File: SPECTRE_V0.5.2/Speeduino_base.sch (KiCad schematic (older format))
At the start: 218 parts, among them J1 Conn_01x06_Male, J2 Conn_02x04_Odd_Even, J3 ProtoArea, Q1 AO3400, Q10 BSP78, Q11 BSP78, Q12 AO3400, Q13 BSP78, Q14 BSP78, Q15 BSP78, Q16 BSP78, Q17 BSP78, Q18 BSP78, Q19 BSP78, Q20 BSP78, Q21 BSP78, Q6 AO3400, Q7 AO3400, Q8 AO3400, Q9 AO3400, U1 MAX9926UAEE+, U2 LM78M05_TO220, U3 TL431DBZ, U4 molex_48pin, U5 TJA1050, U6 MAX3232, U7 MIC4427, U8 MIC4427, U9 MIC4427

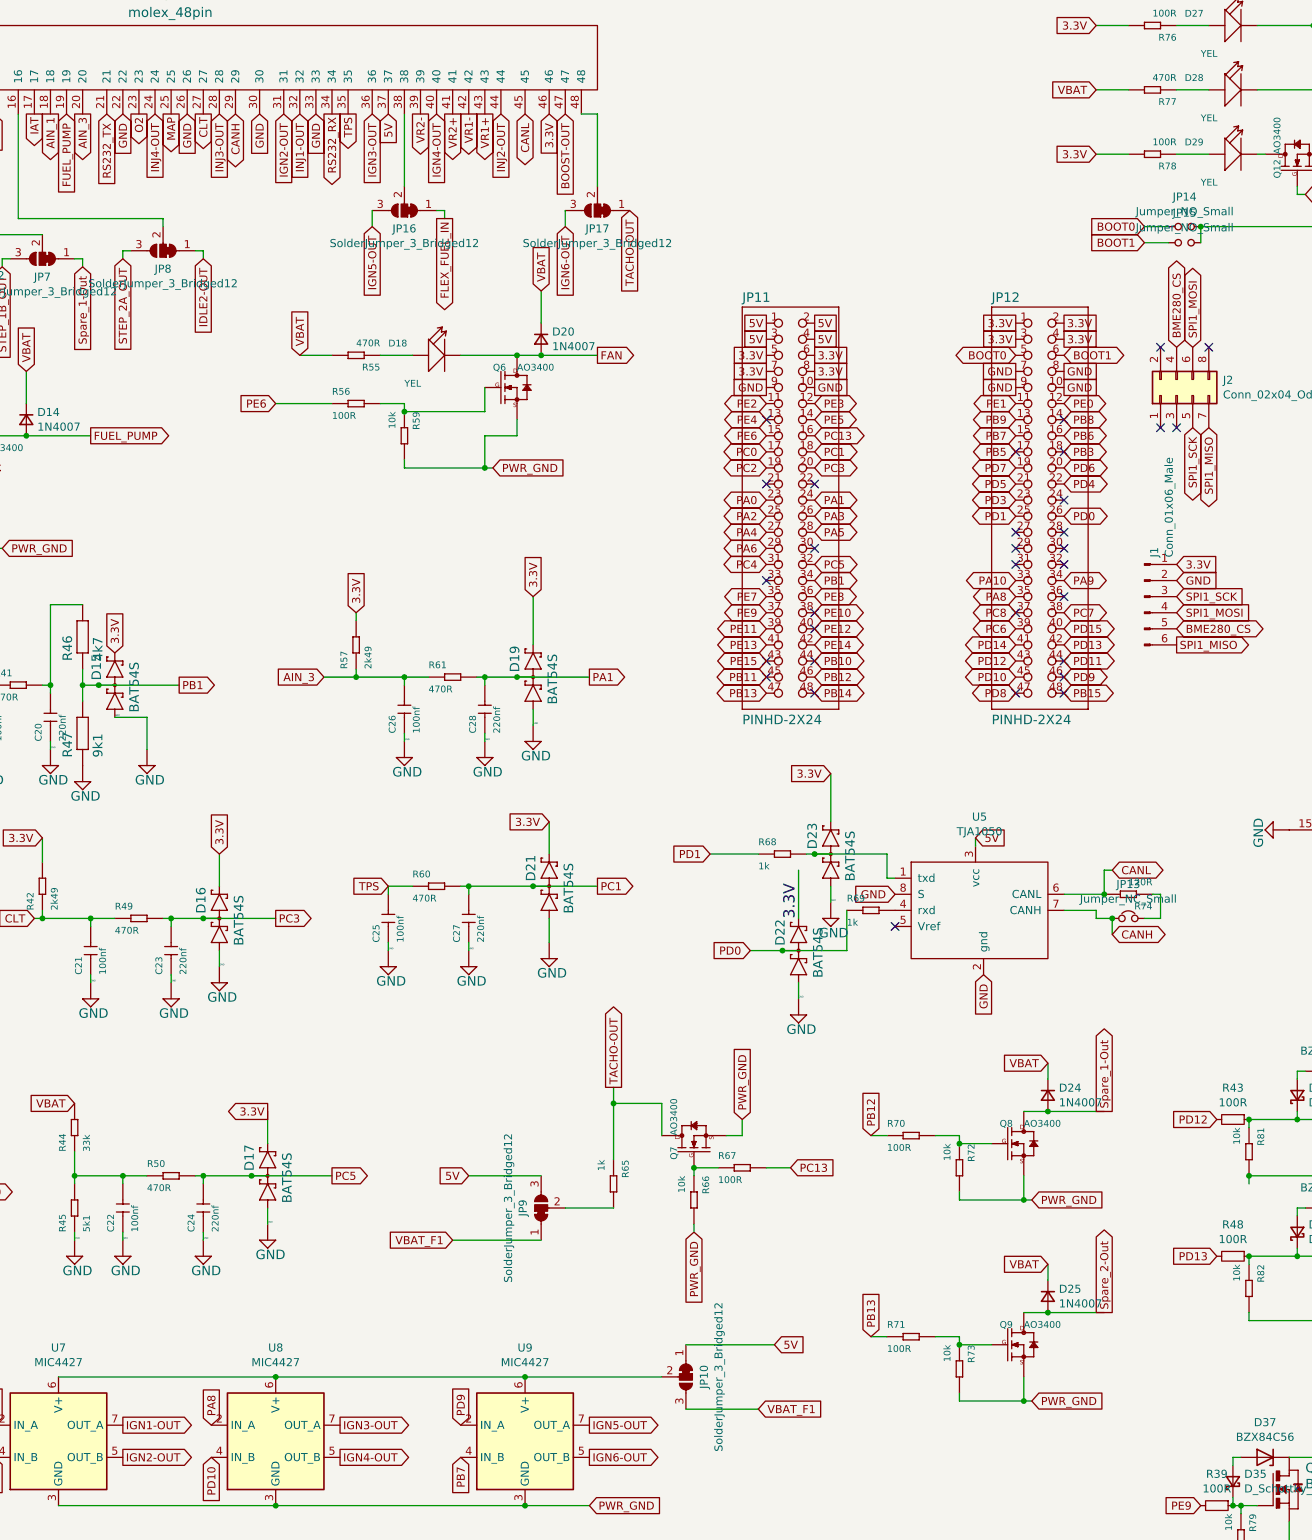
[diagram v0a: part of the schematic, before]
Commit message: Updates on V0.5.2
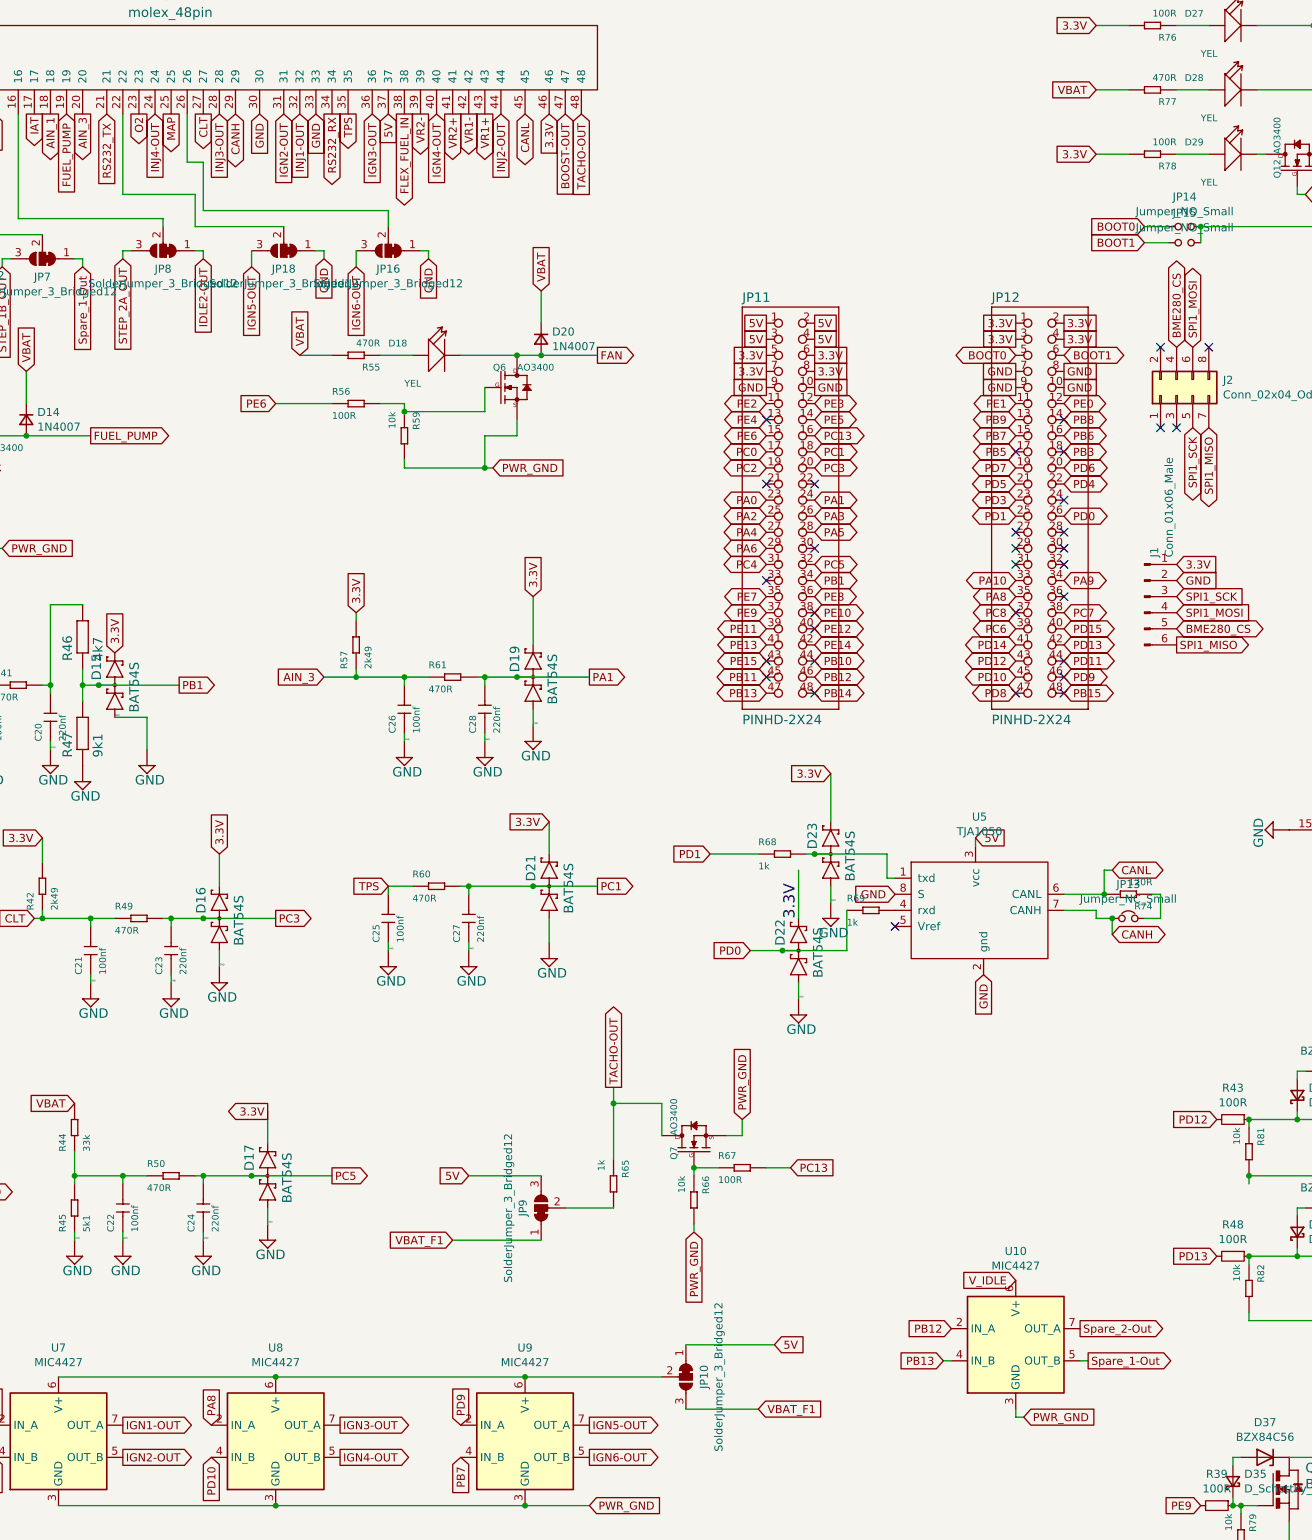
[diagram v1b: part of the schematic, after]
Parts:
- removed D24, D25: 1N4007, Diode_SMD:D_SMA, symbol Device:D_Small
- removed JP17: SolderJumper_3_Bridged12, Jumper:SolderJumper-3_P1.3mm_Bridged12_Pad1.0x1.5mm, symbol Jumper:SolderJumper_3_Bridged12
- removed Q8, Q9: AO3400, Speeduino_base:SOT-23, symbol Speeduino_base-eagle-import:SMD-MOSFET-N-CH-20V-2.1A-CJ2302(SOT-23)
- removed R70, R71: 100R, Speeduino_base:R0603, symbol Speeduino_base-eagle-import:SMD-RES-470R-5%-1_10W(0603)
- removed R72, R73: 10k, Speeduino_base:R0603, symbol Speeduino_base-eagle-import:SMD-RES-470R-5%-1_10W(0603)
- added JP18: SolderJumper_3_Bridged12, Jumper:SolderJumper-3_P1.3mm_Bridged12_Pad1.0x1.5mm, symbol Jumper:SolderJumper_3_Bridged12
- added U10: MIC4427, Package_SO:SO-8_3.9x4.9mm_P1.27mm, symbol Driver_FET:MIC4427
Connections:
- net FLEX_FUEL_IN: now also U4.38; no longer JP16.1 (A)
- net GND: now also JP16.1 (A), JP18.1 (A); no longer U4.22, U4.26
- net IGN5-OUT: now also JP18.3 (B); no longer JP16.3 (B)
- net IGN6-OUT: now also JP16.3 (B)
- net PB12: now also U10.2 (IN_A)
- net PB13: now also U10.4 (IN_B)
- net PWR_GND: now also U10.3 (GND)
- net Spare_1-Out: now also U10.5 (OUT_B)
- net Spare_2-Out: now also U10.7 (OUT_A)
- net TACHO-OUT: now also U4.48
- net V_IDLE: now also U10.6 (V+)
- net at JP16.2 (C): now also U4.26; no longer U4.38
- new net: JP18.2 (C), U4.22
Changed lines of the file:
@@
 Text GLabel 6500 1400 3    50   Output ~ 0
 MAP
-Text GLabel 6600 1400 3    50   Input ~ 0
-GND
 Text GLabel 5650 1400 3    50   Output ~ 0
 IAT
@@
 Text GLabel 8850 1400 3    50   Input ~ 0
 3.3V
-Text GLabel 8200 2050 3    50   Output ~ 0
+Text GLabel 7950 1400 3    50   Output ~ 0
 FLEX_FUEL_IN
-Text GLabel 9350 2000 3    50   Input ~ 0
-TACHO-OUT
 $Comp
 L Jumper:SolderJumper_3_Bridged12 JP8
@@
 Wire Wire Line
 	750  10300 750  10400
-Text GLabel 6200 1400 3    50   Input ~ 0
+Text GLabel 7450 2300 3    50   Input ~ 0
 GND
 Text GLabel 7050 1400 3    50   Input ~ 0
@@
 Wire Wire Line
 	4050 11100 4050 11200
-Text GLabel 11850 9400 2    50   Input ~ 0
+Text GLabel 11800 9500 2    50   Input ~ 0
 PWR_GND
-Text GLabel 12300 8850 1    50   Output ~ 0
+Text GLabel 12150 8950 2    50   Output ~ 0
 Spare_2-Out
-Text GLabel 11950 8550 0    50   Input ~ 0
-VBAT
-Wire Wire Line
-	11400 9400 11800 9400
-Wire Wire Line
-	11400 9050 11600 9050
-Wire Wire Line
-	11250 9000 11400 9000
-Wire Wire Line
-	11400 9000 11400 9050
-Connection ~ 11400 9050
-Wire Wire Line
-	11400 9350 11400 9400
-Wire Wire Line
-	11800 9400 11800 9250
-Wire Wire Line
-	11800 8850 11950 8850
-$Comp
-L Speeduino_base-eagle-import:SMD-RES-470R-5%-1_10W(0603) R73
-U 1 1 5F3D9256
-P 11400 9200
-F 0 "R73" H 11250 9250 42  0000 L BNN
-F 1 "10k" H 11250 9100 42  0000 L BNN
-F 2 "Speeduino_base:R0603" H 11400 9200 50  0001 C CNN
-F 3 "" H 11400 9200 50  0001 C CNN
-	1    11400 9200
-	0    1    1    0
-$EndComp
-$Comp
-L Speeduino_base-eagle-import:SMD-RES-470R-5%-1_10W(0603) R71
-U 1 1 5F3D9262
-P 11100 9000
-F 0 "R71" H 10950 9050 42  0000 L BNN
-F 1 "100R" H 10950 8900 42  0000 L BNN
-F 2 "Speeduino_base:R0603" H 11100 9000 50  0001 C CNN
-F 3 "" H 11100 9000 50  0001 C CNN
-	1    11100 9000
-	1    0    0    -1
-$EndComp
-$Comp
-L Speeduino_base-eagle-import:SMD-MOSFET-N-CH-20V-2.1A-CJ2302(SOT-23) Q9
-U 1 1 5F3D9268
-P 11800 9050
-F 0 "Q9" H 11650 9150 42  0000 L BNN
-F 1 "AO3400" H 11800 9150 42  0000 L BNN
-F 2 "Speeduino_base:SOT-23" H 11800 9050 50  0001 C CNN
-F 3 "" H 11800 9050 50  0001 C CNN
-	1    11800 9050
-	1    0    0    -1
-$EndComp
-$Comp
-L Device:D_Small D25
-U 1 1 5F3D926E
-P 11950 8750
-F 0 "D25" V 11904 8818 50  0000 L CNN
-F 1 "1N4007" V 11995 8818 50  0000 L CNN
-F 2 "Diode_SMD:D_SMA" V 11950 8750 50  0001 C CNN
-F 3 "~" V 11950 8750 50  0001 C CNN
-	1    11950 8750
-	0    1    1    0
-$EndComp
-Wire Wire Line
-	11950 8850 12300 8850
-Connection ~ 11950 8850
-Text GLabel 10850 9000 1    50   Input ~ 0
+Text GLabel 11750 8650 0    50   Input ~ 0
+V_IDLE
+Text GLabel 11300 9150 0    50   Input ~ 0
 PB13
-Wire Wire Line
-	10850 9000 10950 9000
-Wire Wire Line
-	11850 9400 11800 9400
-Connection ~ 11800 9400
-Wire Wire Line
-	11950 8550 11950 8650
-Text GLabel 11850 8150 2    50   Input ~ 0
-PWR_GND
-Text GLabel 12300 7600 1    50   Output ~ 0
+Text GLabel 12200 9150 2    50   Output ~ 0
 Spare_1-Out
-Text GLabel 11950 7300 0    50   Input ~ 0
-VBAT
-Wire Wire Line
-	11400 8150 11800 8150
-Wire Wire Line
-	11400 7800 11600 7800
-Wire Wire Line
-	11250 7750 11400 7750
-Wire Wire Line
-	11400 7750 11400 7800
-Connection ~ 11400 7800
-Wire Wire Line
-	11400 8100 11400 8150
-Wire Wire Line
-	11800 8150 11800 8000
-Wire Wire Line
-	11800 7600 11950 7600
-$Comp
-L Speeduino_base-eagle-import:SMD-RES-470R-5%-1_10W(0603) R72
-U 1 1 5F7FAD08
-P 11400 7950
-F 0 "R72" H 11250 8000 42  0000 L BNN
-F 1 "10k" H 11250 7850 42  0000 L BNN
-F 2 "Speeduino_base:R0603" H 11400 7950 50  0001 C CNN
-F 3 "" H 11400 7950 50  0001 C CNN
-	1    11400 7950
-	0    1    1    0
-$EndComp
-$Comp
-L Speeduino_base-eagle-import:SMD-RES-470R-5%-1_10W(0603) R70
-U 1 1 5F7FAD0E
-P 11100 7750
-F 0 "R70" H 10950 7800 42  0000 L BNN
-F 1 "100R" H 10950 7650 42  0000 L BNN
-F 2 "Speeduino_base:R0603" H 11100 7750 50  0001 C CNN
-F 3 "" H 11100 7750 50  0001 C CNN
-	1    11100 7750
-	1    0    0    -1
-$EndComp
-$Comp
-L Speeduino_base-eagle-import:SMD-MOSFET-N-CH-20V-2.1A-CJ2302(SOT-23) Q8
-U 1 1 5F7FAD14
-P 11800 7800
-F 0 "Q8" H 11650 7900 42  0000 L BNN
-F 1 "AO3400" H 11800 7900 42  0000 L BNN
-F 2 "Speeduino_base:SOT-23" H 11800 7800 50  0001 C CNN
-F 3 "" H 11800 7800 50  0001 C CNN
-	1    11800 7800
-	1    0    0    -1
-$EndComp
-$Comp
-L Device:D_Small D24
-U 1 1 5F7FAD1A
-P 11950 7500
-F 0 "D24" V 11904 7568 50  0000 L CNN
-F 1 "1N4007" V 11995 7568 50  0000 L CNN
-F 2 "Diode_SMD:D_SMA" V 11950 7500 50  0001 C CNN
-F 3 "~" V 11950 7500 50  0001 C CNN
-	1    11950 7500
-	0    1    1    0
-$EndComp
-Wire Wire Line
-	11950 7600 12300 7600
-Connection ~ 11950 7600
-Text GLabel 10850 7750 1    50   Input ~ 0
+Text GLabel 11350 8950 0    50   Input ~ 0
 PB12
-Wire Wire Line
-	10850 7750 10950 7750
-Wire Wire Line
-	11850 8150 11800 8150
-Connection ~ 11800 8150
-Wire Wire Line
-	11950 7300 11950 7400
 Text GLabel 16450 10950 2    50   Output ~ 0
 INJ8-OUT
@@
 Connection ~ 7150 10050
 Connection ~ 8700 10050
-$Comp
-L Jumper:SolderJumper_3_Bridged12 JP16
-U 1 1 5F69F1FE
-P 7950 2000
-F 0 "JP16" H 7950 2113 50  0000 C CNN
-F 1 "SolderJumper_3_Bridged12" H 7950 2204 50  0000 C CNN
-F 2 "Jumper:SolderJumper-3_P1.3mm_Bridged12_Pad1.0x1.5mm" H 7950 2000 50  0001 C CNN
-F 3 "~" H 7950 2000 50  0001 C CNN
-	1    7950 2000
-	-1   0    0    1
-$EndComp
-Text GLabel 7750 2100 3    50   Input ~ 0
-IGN5-OUT
-Wire Wire Line
-	7750 2000 7750 2100
-Wire Wire Line
-	8150 2000 8200 2000
-Wire Wire Line
-	8200 2000 8200 2050
-Wire Wire Line
-	7950 1400 7950 1850
-$Comp
-L Jumper:SolderJumper_3_Bridged12 JP17
-U 1 1 5F83750C
-P 9150 2000
-F 0 "JP17" H 9150 2113 50  0000 C CNN
-F 1 "SolderJumper_3_Bridged12" H 9150 2204 50  0000 C CNN
-F 2 "Jumper:SolderJumper-3_P1.3mm_Bridged12_Pad1.0x1.5mm" H 9150 2000 50  0001 C CNN
-F 3 "~" H 9150 2000 50  0001 C CNN
-	1    9150 2000
-	-1   0    0    1
-$EndComp
-Text GLabel 8950 2100 3    50   Input ~ 0
-IGN6-OUT
-Wire Wire Line
-	8950 2000 8950 2100
-Wire Wire Line
-	9150 1850 9150 1400
-Wire Wire Line
-	9150 1400 9050 1400
 Text GLabel 7450 11050 3    50   Input ~ 0
 5V
@@
 Text GLabel 2600 2350 3    50   Input ~ 0
 5V
+$Comp
+L Jumper:SolderJumper_3_Bridged12 JP18
+U 1 1 5F36B798
+P 7200 2250
+F 0 "JP18" H 7200 2363 50  0000 C CNN
+F 1 "SolderJumper_3_Bridged12" H 7200 2454 50  0000 C CNN
+F 2 "Jumper:SolderJumper-3_P1.3mm_Bridged12_Pad1.0x1.5mm" H 7200 2250 50  0001 C CNN
+F 3 "~" H 7200 2250 50  0001 C CNN
+	1    7200 2250
+	-1   0    0    1
+$EndComp
+Text GLabel 7000 2350 3    50   Input ~ 0
+IGN5-OUT
+Wire Wire Line
+	7000 2250 7000 2350
+Wire Wire Line
+	7400 2250 7450 2250
+Wire Wire Line
+	7450 2250 7450 2300
+Wire Wire Line
+	7200 2100 6650 2100
+Wire Wire Line
+	6650 2100 6650 1900
+Wire Wire Line
+	6650 1900 6200 1900
+Wire Wire Line
+	6200 1900 6200 1400
+Text GLabel 9050 1400 3    50   Input ~ 0
+TACHO-OUT
+Text GLabel 8100 2300 3    50   Input ~ 0
+GND
+$Comp
+L Jumper:SolderJumper_3_Bridged12 JP16
+U 1 1 5F462689
+P 7850 2250
+F 0 "JP16" H 7850 2363 50  0000 C CNN
+F 1 "SolderJumper_3_Bridged12" H 7850 2454 50  0000 C CNN
+F 2 "Jumper:SolderJumper-3_P1.3mm_Bridged12_Pad1.0x1.5mm" H 7850 2250 50  0001 C CNN
+F 3 "~" H 7850 2250 50  0001 C CNN
+	1    7850 2250
+	-1   0    0    1
+$EndComp
+Text GLabel 7650 2350 3    50   Input ~ 0
+IGN6-OUT
+Wire Wire Line
+	7650 2250 7650 2350
+Wire Wire Line
+	8050 2250 8100 2250
+Wire Wire Line
+	8100 2250 8100 2300
+Wire Wire Line
+	7850 2100 7850 2000
+Wire Wire Line
+	7850 2000 6700 2000
+Wire Wire Line
+	6700 2000 6700 1700
+Wire Wire Line
+	6700 1700 6600 1700
+Wire Wire Line
+	6600 1700 6600 1400
+$Comp
+L Driver_FET:MIC4427 U10
+U 1 1 5F558FC7
+P 11750 9050
+F 0 "U10" H 11750 9631 50  0000 C CNN
+F 1 "MIC4427" H 11750 9540 50  0000 C CNN
+F 2 "Package_SO:SO-8_3.9x4.9mm_P1.27mm" H 11750 8750 50  0001 C CNN
+F 3 "http://ww1.microchip.com/downloads/en/DeviceDoc/mic4426.pdf" H 11750 8750 50  0001 C CNN
+	1    11750 9050
+	1    0    0    -1
+$EndComp
+Wire Wire Line
+	11750 9450 11750 9500
+Wire Wire Line
+	11750 9500 11800 9500
+Wire Wire Line
+	11350 9150 11300 9150
+Wire Wire Line
+	12150 9150 12200 9150
 $EndSCHEMATC
